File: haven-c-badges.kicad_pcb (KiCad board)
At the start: 2 copper layers, 61.3 x 97 mm, 14 parts, among them U1 NT3H2111W0FHKH

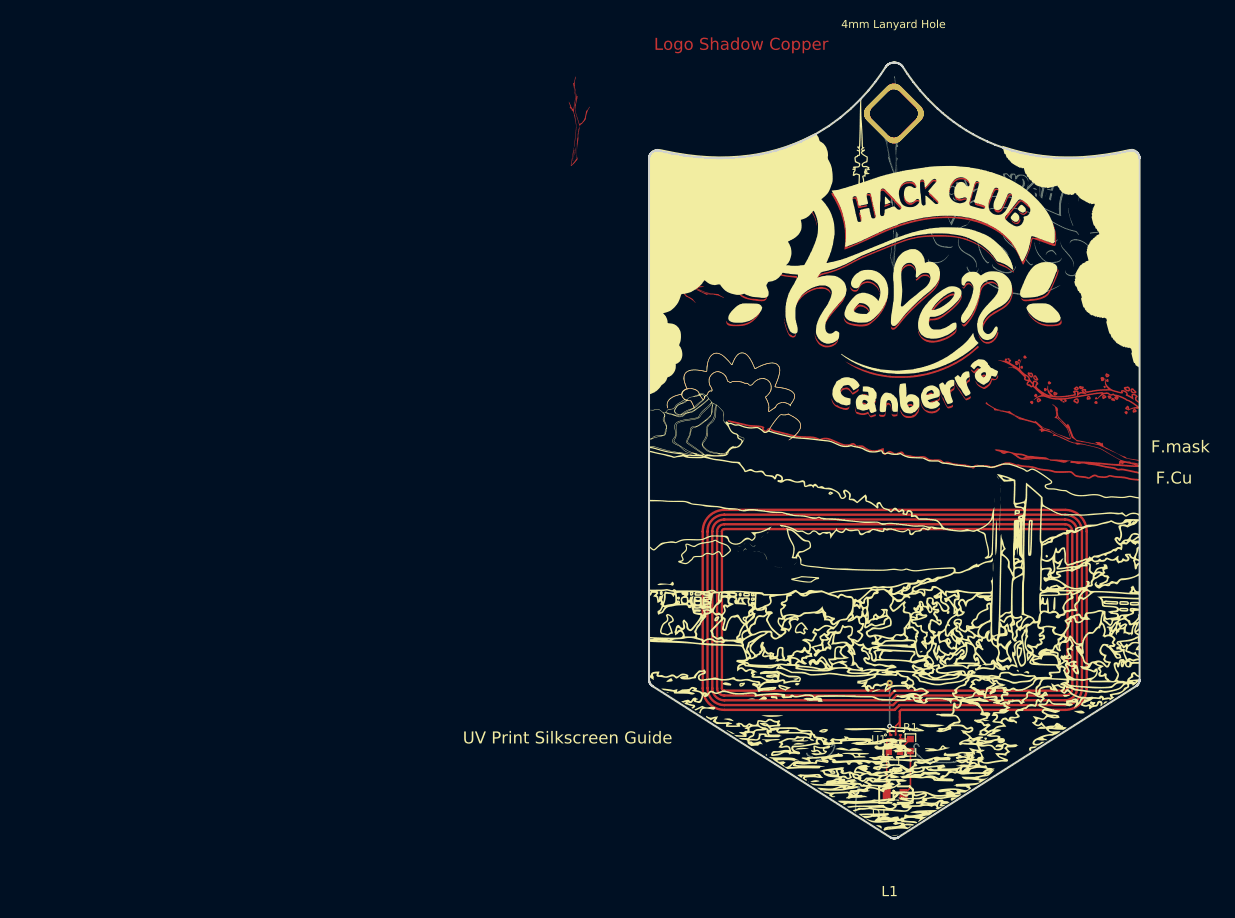
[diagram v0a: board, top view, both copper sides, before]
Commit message: new gerbers pls work (incl ref pictures)
also embedded the img in the kicad pcb
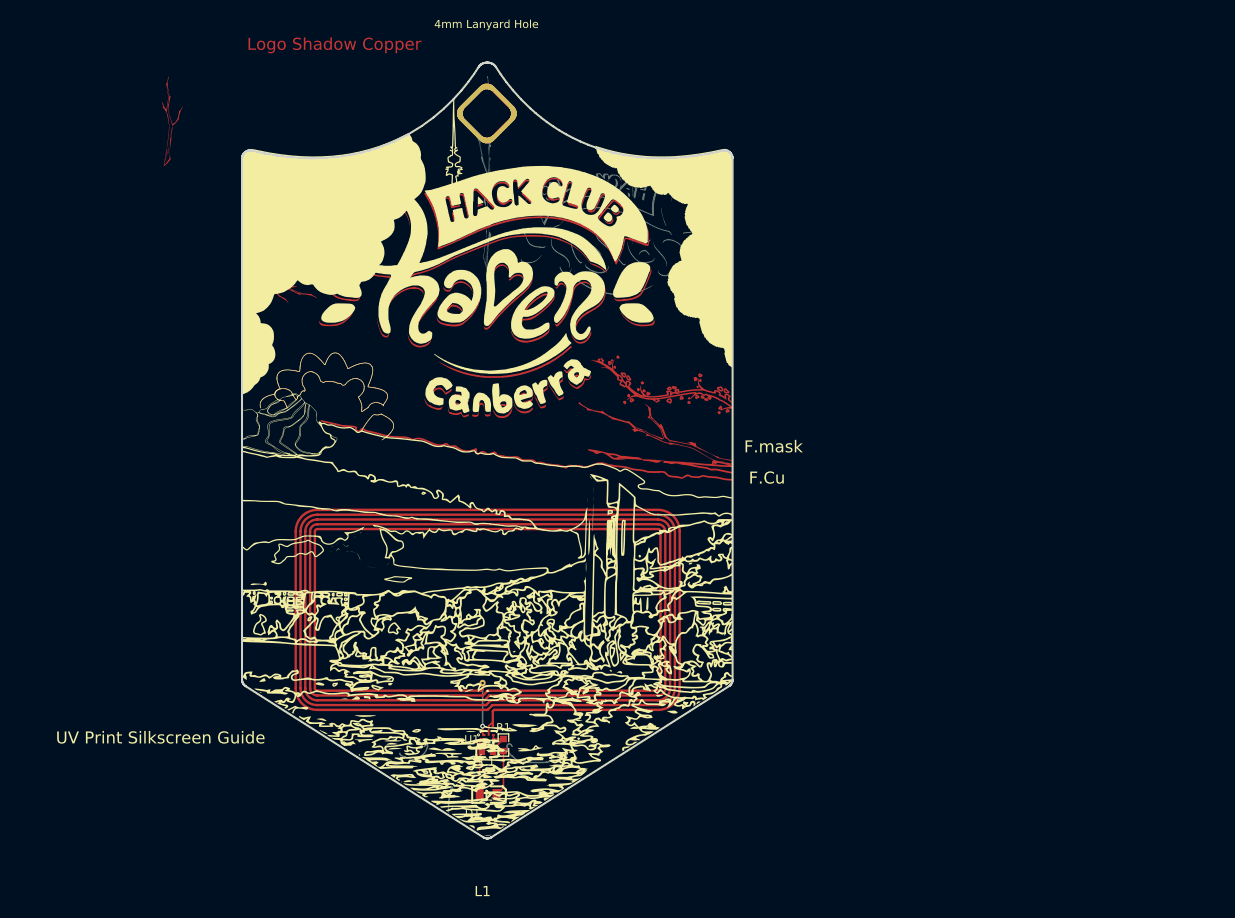
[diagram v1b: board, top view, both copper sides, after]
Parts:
- moved 4mm Lanyard Hole 50.9 mm to (126.6, 54.1)
- moved C1 50.9 mm to (126.7, 133.9)
- moved D1 50.9 mm to (126.8, 139.3)
- moved F.mask 50.9 mm to (126.7, 95.5)
- moved Logo Copper 50.9 mm to (143.7, 70.3)
- moved Logo Mask 50.9 mm to (143.7, 70.2)
- moved Logo Shadow Copper 50.9 mm to (126.6, 76.5)
- moved LogoShadowMask 50.9 mm to (126.6, 76.5)
- moved R1 50.9 mm to (128.7, 133.1)
- moved U1 50.9 mm to (126.8, 132.3)
- moved B.Silkscreen 50.9 mm to (126.7, 95.3)
- moved F.Cu 50.9 mm to (126.7, 95.5)
- moved L1 50.9 mm to (126.7, 116.2)
- moved UV Print Silkscreen Guide 50.9 mm to (126.7, 95.5)
